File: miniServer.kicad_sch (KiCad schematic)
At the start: 28 parts, among them J10 Conn_01x01, J3 Conn_ARM_SWD_TagConnect_TC203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, U1 STM32H725VGTx

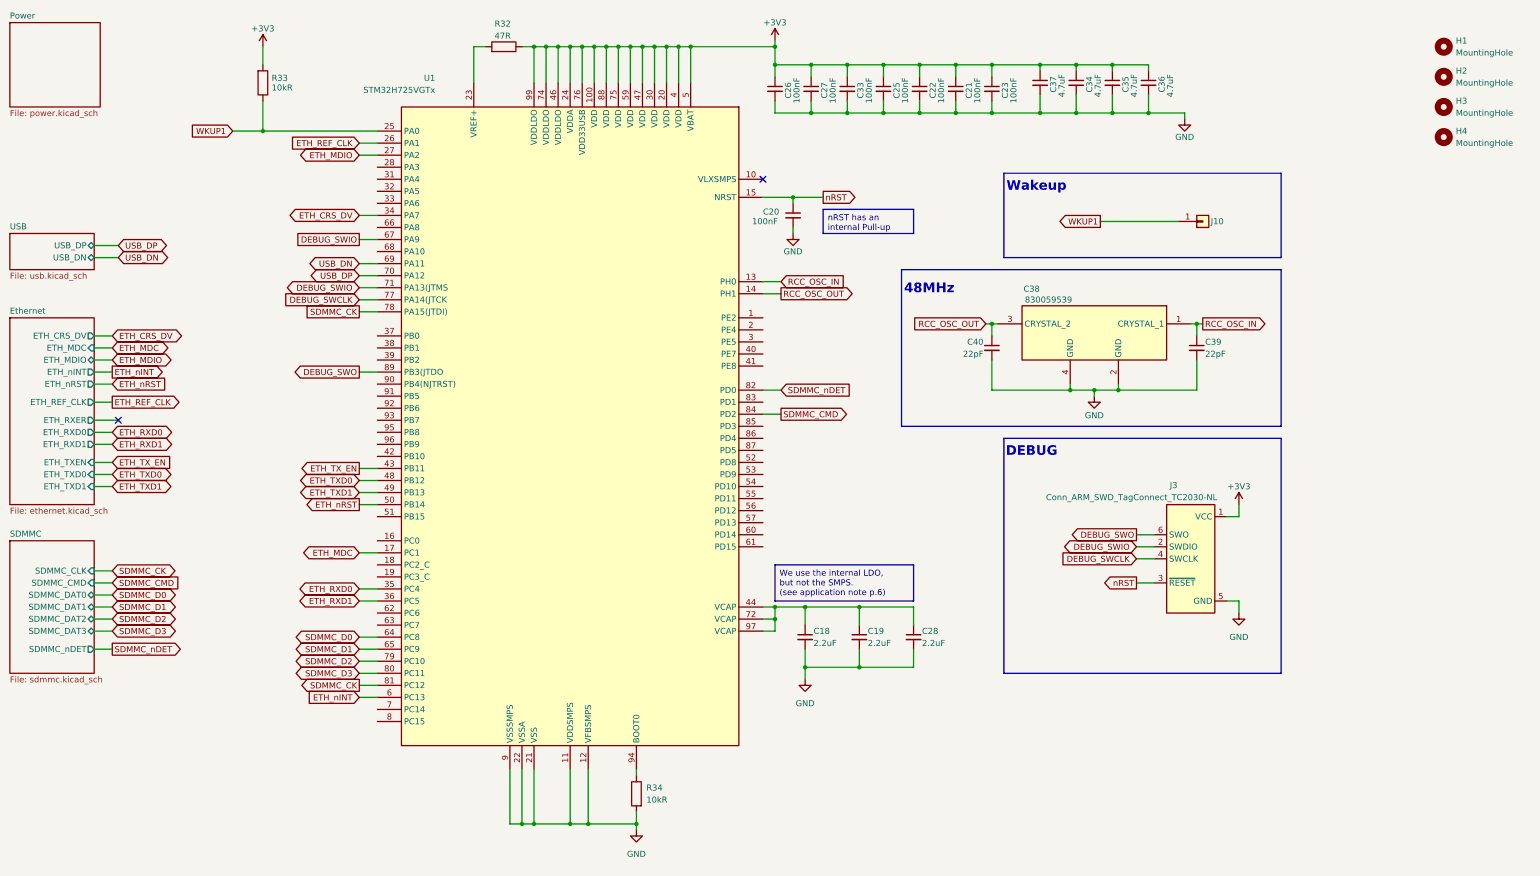
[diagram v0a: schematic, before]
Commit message: Started layout v2
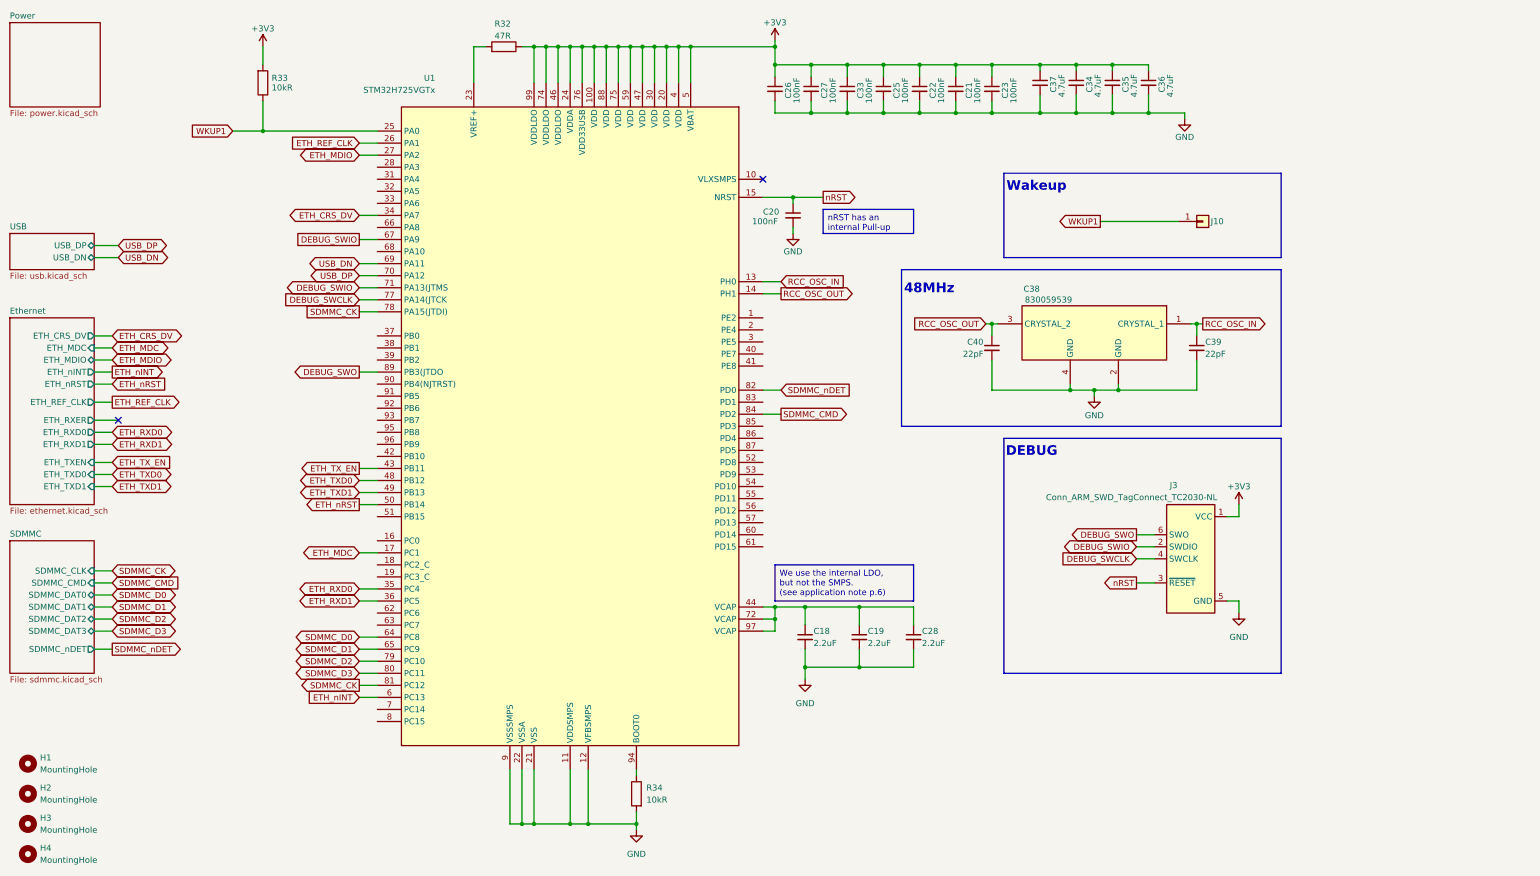
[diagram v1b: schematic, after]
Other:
- moved on the sheet: H1, H2, H3, H4
